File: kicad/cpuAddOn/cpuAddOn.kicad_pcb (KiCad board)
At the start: 6 copper layers, 60.6 x 100 mm, 141 parts, among them J1 QTE-020-01-X-D-A, J2 105450-0101, J3 Conn_01x05_Pin, J4 SJ-3551B-MSMT-TR-67, J5 TE_2311765-1, J7 Conn_02x16_Odd_Even, SW1 B3U-1000P[], SW2 B3U-1000P[], SW3 B3U-1000P[], SW4 B3U-1000P[], SW5 B3U-1000P[], U1 USB2513B-AEZC, U10 MAX9867ETJ+, U11 LP5907MFX-1.8, U12 MX25R3235FM2IL0, U13 ICM-42605, U14 SHT40-AD1B-R2, U15 TCS34003FNM, U16 HDSM-433C, U2 NCP1529A, U3 STM32F103CBU6, U4 SN74HC266DR, U5 AP2281-3WG-7, U6 STM32H743ZITx, U7 AS4C16M16SA-6TAN, U8 ISO1044BD, U9 TS3A227ERVAR, X1 ECS-2520MV-240-BL-TR, X2 ECS-2520MV-080-BM-TR, Y1 RT2012-32.768-9-20-EXT-TR

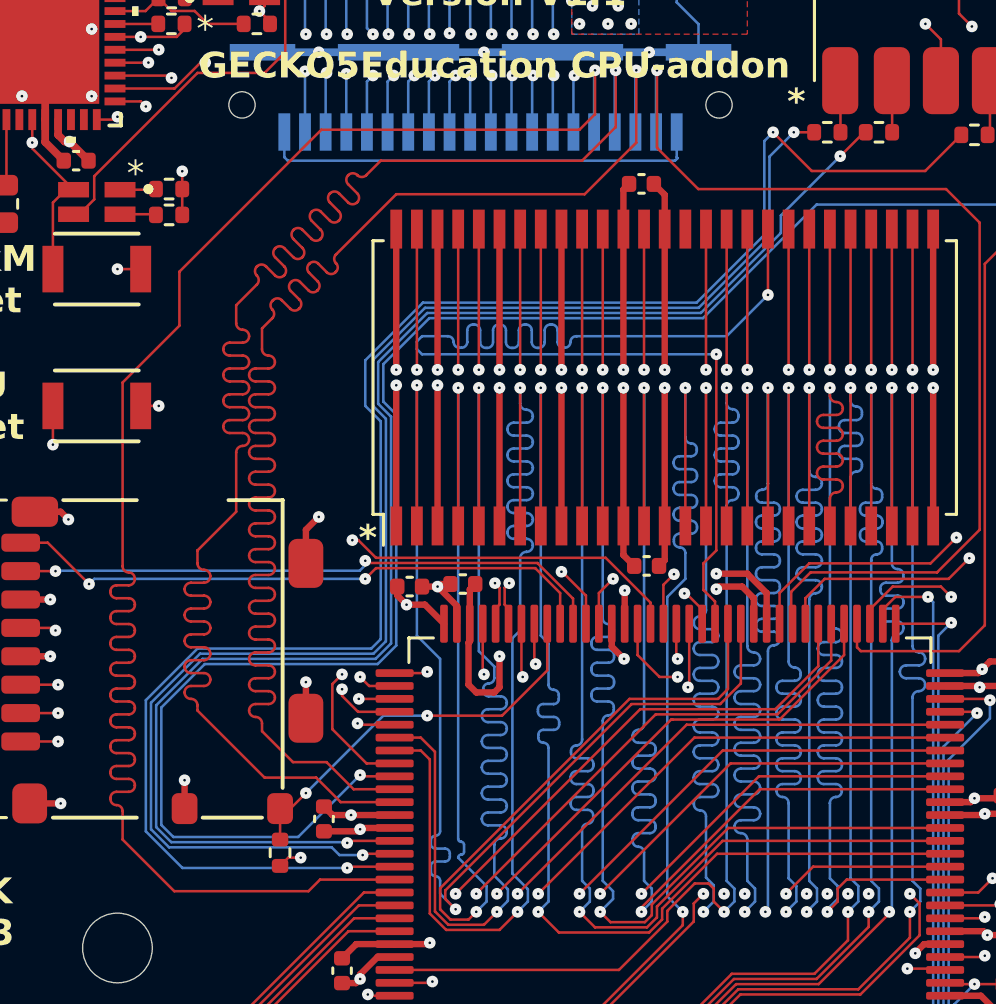
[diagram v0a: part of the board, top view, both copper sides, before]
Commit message: Made an alternative version
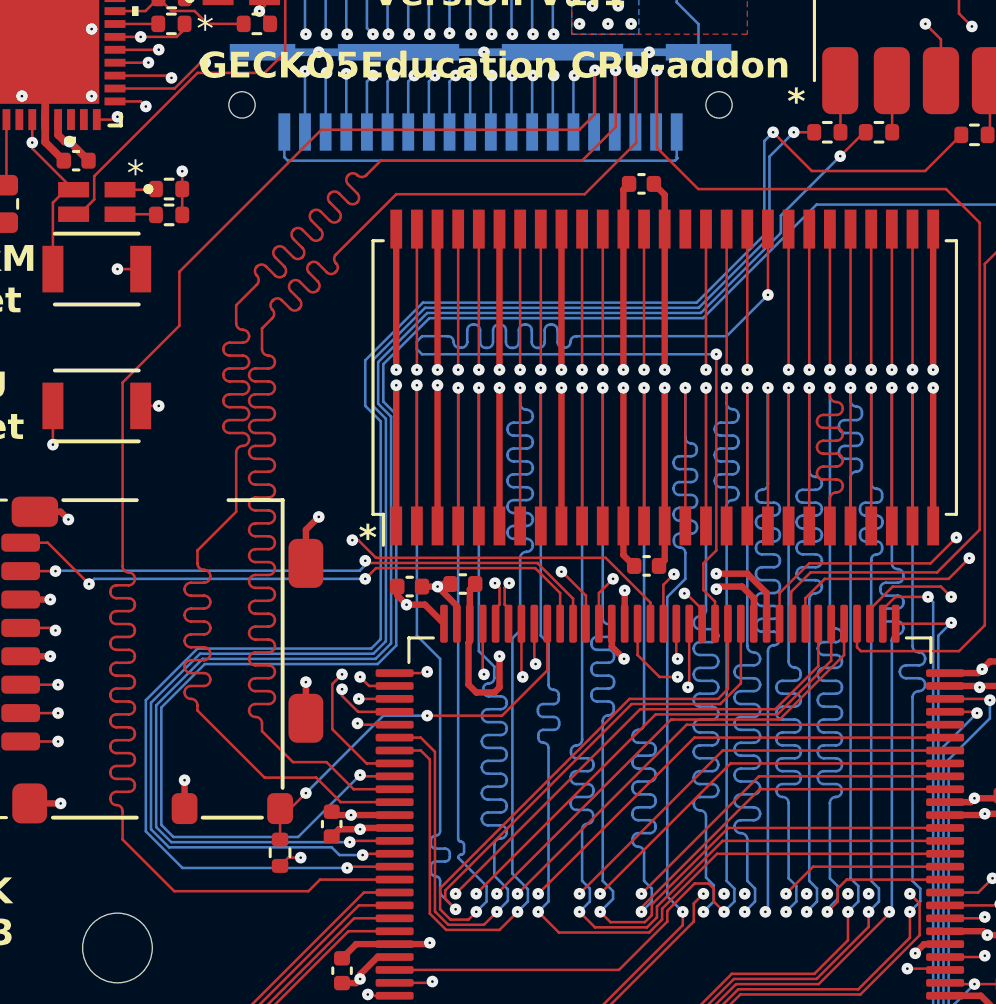
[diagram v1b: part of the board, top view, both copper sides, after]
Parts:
- moved C42 0.36 mm to (106.8, 94.6)
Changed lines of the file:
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@@
   )
   (footprint "Capacitor_SMD:C_0402_1005Metric" (layer "F.Cu")
-    (at 106.5 94.4 90)
+    (at 106.8 94.6 90)
     (descr "Capacitor SMD 0402 (1005 Metric), square (rectangular) end terminal, IPC_7351 nominal, (Body size source: IPC-SM-782 page 76, https://www.pcb-3d.com/wordpress/wp-content/uploads/ipc-sm-782a_amendment_1_and_2.pdf), generated with kicad-footprint-generator")
     (tags "capacitor")
@@
   (segment (start 107.8275 112.43) (end 107.8075 112.45) (width 0.25) (layer "F.Cu") (net 1))
   (segment (start 130.5625 98.75) (end 132.05 98.75) (width 0.25) (layer "F.Cu") (net 1))
-  (segment (start 106.5 94.88) (end 107.82 94.88) (width 0.25) (layer "F.Cu") (net 1))
   (segment (start 109.2375 105.75) (end 109.2375 106.25) (width 0.25) (layer "F.Cu") (net 1))
   (segment (start 107.8275 111.9) (end 107.8275 112.43) (width 0.25) (layer "F.Cu") (net 1))
@@
   (segment (start 91.7 120.7836) (end 91.455 120.5386) (width 0.2) (layer "F.Cu") (net 1))
   (segment (start 104.8 41.08) (end 105.78 41.08) (width 0.1) (layer "F.Cu") (net 1))
+  (segment (start 107.9 94.8) (end 107.08 94.8) (width 0.25) (layer "F.Cu") (net 1))
   (segment (start 119.7 84.38) (end 119.48 84.6) (width 0.25) (layer "F.Cu") (net 1))
   (segment (start 107.300001 49.3896) (end 107.300001 51.139999) (width 0.25) (layer "F.Cu") (net 1))
@@
   (segment (start 125.65 108.1625) (end 125.65 110.09) (width 0.25) (layer "F.Cu") (net 1))
   (segment (start 103.655199 48.544801) (end 103.5 48.7) (width 0.25) (layer "F.Cu") (net 1))
+  (segment (start 107.08 94.8) (end 106.8 95.08) (width 0.25) (layer "F.Cu") (net 1))
   (segment (start 110.17 59.57) (end 110.4 59.8) (width 0.1) (layer "F.Cu") (net 1))
   (segment (start 109.2375 99.75) (end 108.575736 99.75) (width 0.25) (layer "F.Cu") (net 1))
@@
   (segment (start 105.44 118.6711) (end 105.04 119.0711) (width 0.25) (layer "F.Cu") (net 1))
   (segment (start 101.7 118.6461) (end 102.685 118.6461) (width 0.25) (layer "F.Cu") (net 1))
-  (segment (start 107.82 94.88) (end 107.9 94.8) (width 0.25) (layer "F.Cu") (net 1))
   (segment (start 101.01 71) (end 101.01 69.31) (width 0.1) (layer "F.Cu") (net 1))
   (segment (start 123.15 85.85) (end 122.7 85.4) (width 0.25) (layer "F.Cu") (net 1))
@@
   (segment (start 104.41 63.6) (end 104.41 63.515) (width 0.1) (layer "F.Cu") (net 11))
   (segment (start 95.700001 67.3088) (end 95.700001 68.180001) (width 0.3) (layer "F.Cu") (net 11))
-  (segment (start 106.5 93.92) (end 106.83 94.25) (width 0.25) (layer "F.Cu") (net 11))
   (segment (start 106.8 41.09) (end 107.77 41.09) (width 0.1) (layer "F.Cu") (net 11))
   (segment (start 120.03 118.705) (end 121.795 118.705) (width 0.3) (layer "F.Cu") (net 11))
@@
   (segment (start 99.6 94.882842) (end 101.017158 96.3) (width 0.1) (layer "B.Cu") (net 94))
   (segment (start 108.334316 87.8) (end 101.6 87.8) (width 0.1) (layer "B.Cu") (net 94))
-  (segment (start 107.4795 95.25) (end 107.4 95.3295) (width 0.1) (layer "F.Cu") (net 95))
+  (segment (start 107.5 95.3) (end 107.55 95.25) (width 0.1) (layer "F.Cu") (net 95))
   (segment (start 127.4255 67.8) (end 126.5 68.7255) (width 0.1) (layer "F.Cu") (net 95))
   (segment (start 127.49 67.8) (end 127.4255 67.8) (width 0.1) (layer "F.Cu") (net 95))
-  (segment (start 109.2375 95.25) (end 107.4795 95.25) (width 0.1) (layer "F.Cu") (net 95))
+  (segment (start 107.55 95.25) (end 109.2375 95.25) (width 0.1) (layer "F.Cu") (net 95))
   (via (at 126.5 68.7255) (size 0.45) (drill 0.1) (layers "F.Cu" "B.Cu") (remove_unused_layers) (keep_end_layers) (zone_layer_connections) (net 95))
-  (via (at 107.4 95.3295) (size 0.45) (drill 0.1) (layers "F.Cu" "B.Cu") (remove_unused_layers) (keep_end_layers) (zone_layer_connections) (net 95))
-  (segment (start 107.4 95.3) (end 107.4 95.3295) (width 0.1) (layer "B.Cu") (net 95))
-  (segment (start 110.5 74.8) (end 108.6 76.7) (width 0.1) (layer "B.Cu") (net 95))
-  (segment (start 100.582842 95.3) (end 107.4 95.3) (width 0.1) (layer "B.Cu") (net 95))
-  (segment (start 124.2 71.7) (end 121.1 74.8) (width 0.1) (layer "B.Cu") (net 95))
-  (segment (start 121.1 74.8) (end 110.5 74.8) (width 0.1) (layer "B.Cu") (net 95))
-  (segment (start 108.6 78.317158) (end 109.1 78.817158) (width 0.1) (layer "B.Cu") (net 95))
-  (segment (start 108.500001 88.2) (end 101.8 88.2) (width 0.1) (layer "B.Cu") (net 95))
-  (segment (start 101.8 88.2) (end 100 90) (width 0.1) (layer "B.Cu") (net 95))
-  (segment (start 109.1 78.817158) (end 109.1 87.600001) (width 0.1) (layer "B.Cu") (net 95))
-  (segment (start 108.6 76.7) (end 108.6 78.317158) (width 0.1) (layer "B.Cu") (net 95))
-  (segment (start 109.1 87.600001) (end 108.500001 88.2) (width 0.1) (layer "B.Cu") (net 95))
-  (segment (start 124.2 71.0255) (end 124.2 71.7) (width 0.1) (layer "B.Cu") (net 95))
-  (segment (start 126.5 68.7255) (end 124.2 71.0255) (width 0.1) (layer "B.Cu") (net 95))
-  (segment (start 100 94.717158) (end 100.582842 95.3) (width 0.1) (layer "B.Cu") (net 95))
-  (segment (start 100 90) (end 100 94.717158) (width 0.1) (layer "B.Cu") (net 95))
+  (via (at 107.5 95.3) (size 0.45) (drill 0.1) (layers "F.Cu" "B.Cu") (remove_unused_layers) (keep_end_layers) (zone_layer_connections) (net 95))
+  (segment (start 110.5 74.8) (end 121.1 74.8) (width 0.1) (layer "B.Cu") (net 95))
+  (segment (start 109.1 78.817158) (end 108.6 78.317158) (width 0.1) (layer "B.Cu") (net 95))
+  (segment (start 100 90) (end 101.8 88.2) (width 0.1) (layer "B.Cu") (net 95))
+  (segment (start 121.1 74.8) (end 124.2 71.7) (width 0.1) (layer "B.Cu") (net 95))
+  (segment (start 100 94.717158) (end 100 90) (width 0.1) (layer "B.Cu") (net 95))
+  (segment (start 108.6 78.317158) (end 108.6 76.7) (width 0.1) (layer "B.Cu") (net 95))
+  (segment (start 101.8 88.2) (end 108.500001 88.2) (width 0.1) (layer "B.Cu") (net 95))
+  (segment (start 108.6 76.7) (end 110.5 74.8) (width 0.1) (layer "B.Cu") (net 95))
+  (segment (start 109.1 87.600001) (end 109.1 78.817158) (width 0.1) (layer "B.Cu") (net 95))
+  (segment (start 108.500001 88.2) (end 109.1 87.600001) (width 0.1) (layer "B.Cu") (net 95))
+  (segment (start 100.582842 95.3) (end 100 94.717158) (width 0.1) (layer "B.Cu") (net 95))
+  (segment (start 107.5 95.3) (end 100.582842 95.3) (width 0.1) (layer "B.Cu") (net 95))
+  (segment (start 124.2 71.0255) (end 126.5 68.7255) (width 0.1) (layer "B.Cu") (net 95))
+  (segment (start 124.2 71.7) (end 124.2 71.0255) (width 0.1) (layer "B.Cu") (net 95))
   (segment (start 126.65 109.45) (end 126.9 109.7) (width 0.25) (layer "F.Cu") (net 96))
   (segment (start 126.65 108.1625) (end 126.65 109.45) (width 0.25) (layer "F.Cu") (net 96))
